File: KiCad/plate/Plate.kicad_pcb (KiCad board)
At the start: 2 copper layers, 133.6 x 74.9 mm, 0 parts

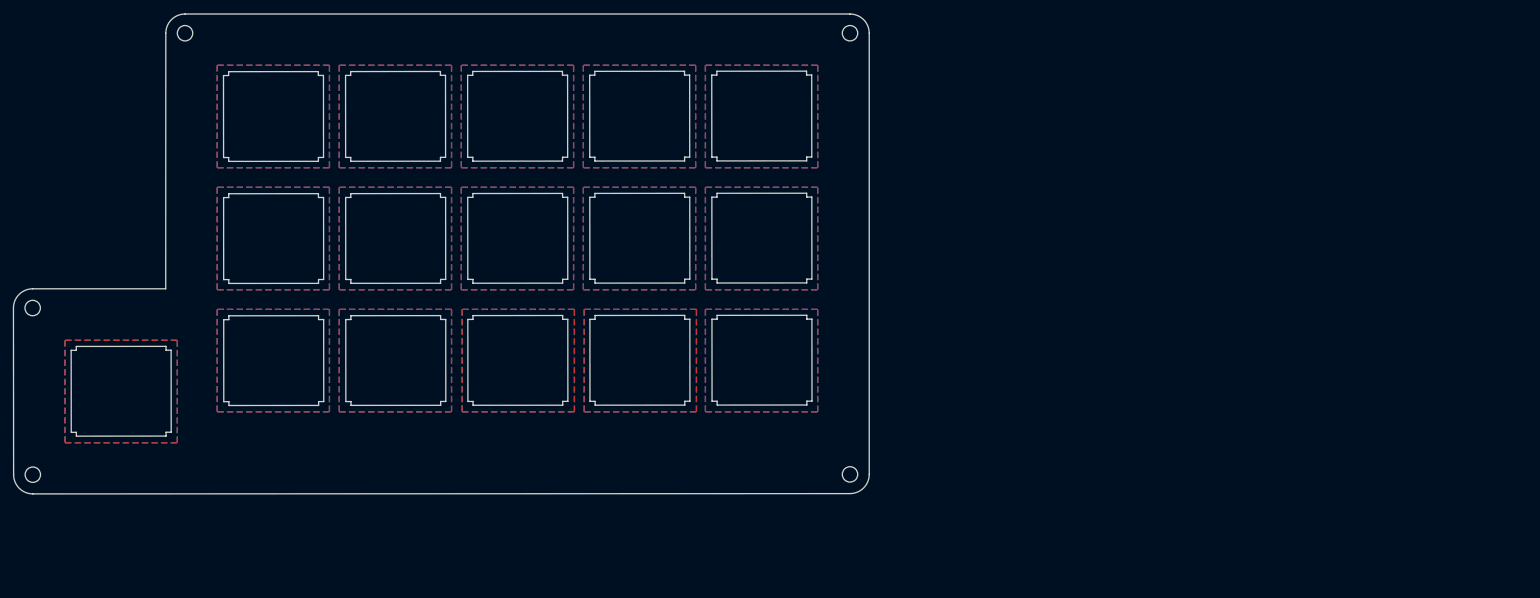
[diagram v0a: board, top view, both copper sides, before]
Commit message: various fixes and changes
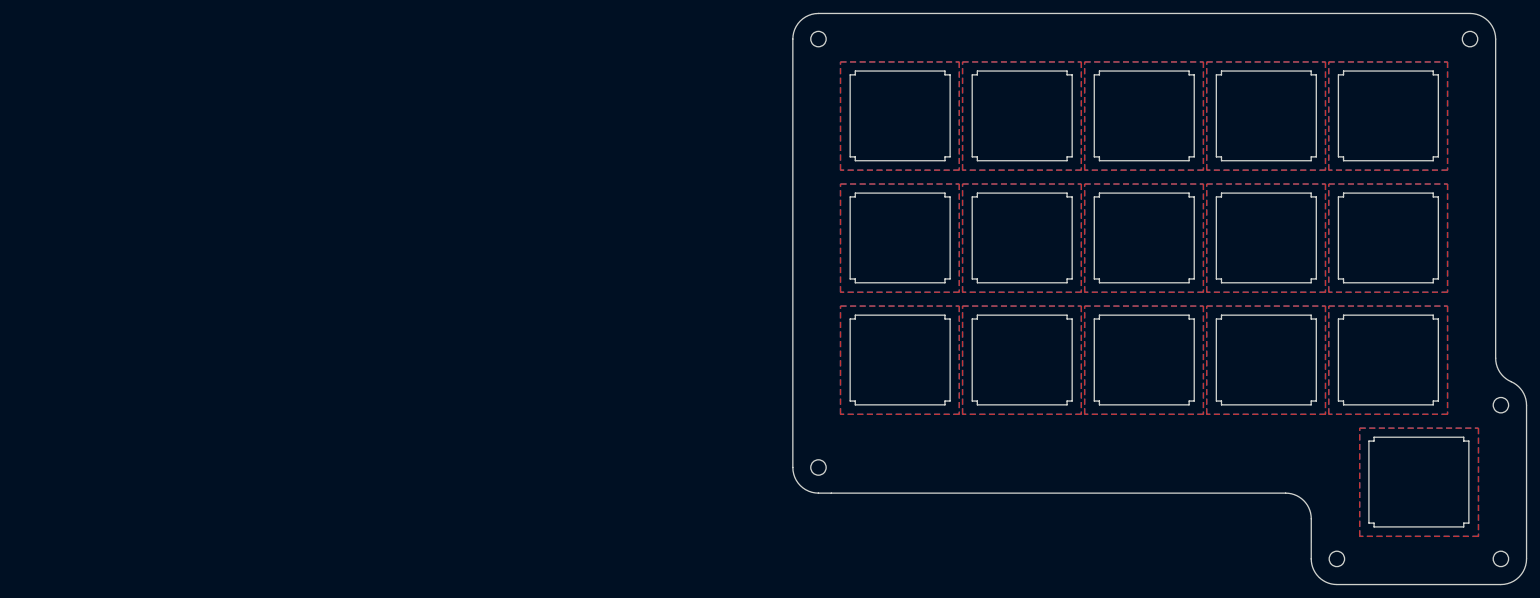
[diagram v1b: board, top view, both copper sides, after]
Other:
- board size 133.6 x 74.9 mm -> 114.5 x 89.1 mm
